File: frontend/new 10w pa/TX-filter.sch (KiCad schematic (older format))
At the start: 48 parts, among them K2 D3002, K3 D3002, K4 D3002, K5 D3002, K6 D3002, P8 CONN_01X08, U3 TPIC6B595, U4 TPIC6B595

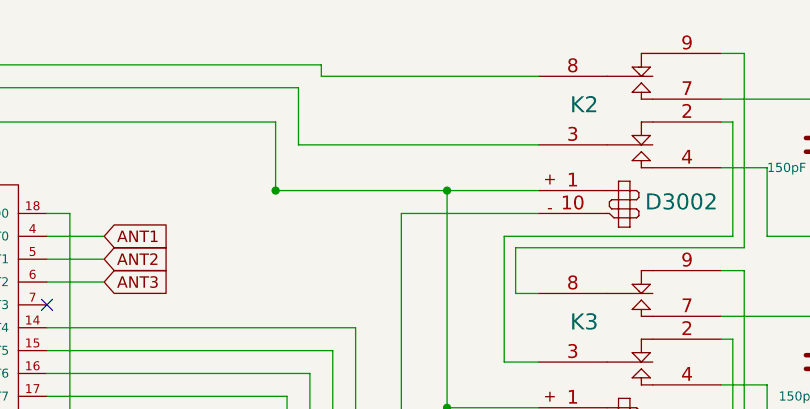
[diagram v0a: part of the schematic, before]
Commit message: More pcb changes
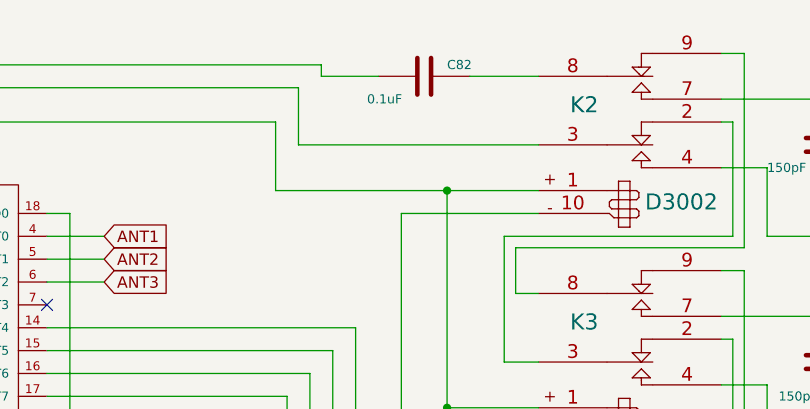
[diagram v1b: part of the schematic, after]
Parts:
- added C82: 0.1uF, HERMESLITE:C_0805, symbol C
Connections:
- net TXIN: now also C82.2; no longer K2.8 (C2)
- new net: C82.1, K2.8 (C2)
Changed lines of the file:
@@
 $EndComp
 $Comp
-L GND #PWR023
+L GND #PWR024
 U 1 1 5496A449
 P 6850 4150
-F 0 "#PWR023" H 6850 4150 30  0001 C CNN
+F 0 "#PWR024" H 6850 4150 30  0001 C CNN
 F 1 "GND" H 6850 4080 30  0001 C CNN
 F 2 "" H 6850 4150 60  0000 C CNN
@@
 $EndComp
 $Comp
-L GND #PWR024
+L GND #PWR025
 U 1 1 5496A44A
 P 5750 4150
-F 0 "#PWR024" H 5750 4150 30  0001 C CNN
+F 0 "#PWR025" H 5750 4150 30  0001 C CNN
 F 1 "GND" H 5750 4080 30  0001 C CNN
 F 2 "" H 5750 4150 60  0000 C CNN
@@
 $EndComp
 $Comp
-L GND #PWR025
+L GND #PWR026
 U 1 1 5496A44B
 P 7750 4150
-F 0 "#PWR025" H 7750 4150 30  0001 C CNN
+F 0 "#PWR026" H 7750 4150 30  0001 C CNN
 F 1 "GND" H 7750 4080 30  0001 C CNN
 F 2 "" H 7750 4150 60  0000 C CNN
@@
 	5400 4400 4400 4400
 $Comp
-L GND #PWR026
+L GND #PWR027
 U 1 1 5496A47D
 P 1900 5550
-F 0 "#PWR026" H 1900 5550 30  0001 C CNN
+F 0 "#PWR027" H 1900 5550 30  0001 C CNN
 F 1 "GND" H 1900 5480 30  0001 C CNN
 F 2 "" H 1900 5550 50  0000 C CNN
@@
 $EndComp
 $Comp
-L GND #PWR027
+L GND #PWR028
 U 1 1 54A155CF
 P 6800 5300
-F 0 "#PWR027" H 6800 5300 30  0001 C CNN
+F 0 "#PWR028" H 6800 5300 30  0001 C CNN
 F 1 "GND" H 6800 5230 30  0001 C CNN
 F 2 "" H 6800 5300 60  0000 C CNN
@@
 $EndComp
 $Comp
-L GND #PWR028
+L GND #PWR029
 U 1 1 54A1568D
 P 7400 5300
-F 0 "#PWR028" H 7400 5300 30  0001 C CNN
+F 0 "#PWR029" H 7400 5300 30  0001 C CNN
 F 1 "GND" H 7400 5230 30  0001 C CNN
 F 2 "" H 7400 5300 60  0000 C CNN
@@
 $EndComp
 $Comp
-L GND #PWR029
+L GND #PWR030
 U 1 1 54A171EB
 P 5950 6400
-F 0 "#PWR029" H 5950 6400 30  0001 C CNN
+F 0 "#PWR030" H 5950 6400 30  0001 C CNN
 F 1 "GND" H 5950 6330 30  0001 C CNN
 F 2 "" H 5950 6400 60  0000 C CNN
@@
 $EndComp
 $Comp
-L GND #PWR030
+L GND #PWR031
 U 1 1 54A171F1
 P 6550 6400
-F 0 "#PWR030" H 6550 6400 30  0001 C CNN
+F 0 "#PWR031" H 6550 6400 30  0001 C CNN
 F 1 "GND" H 6550 6330 30  0001 C CNN
 F 2 "" H 6550 6400 60  0000 C CNN
@@
 $EndComp
 $Comp
-L GND #PWR031
+L GND #PWR032
 U 1 1 54A1B96C
 P 6650 3200
-F 0 "#PWR031" H 6650 3200 30  0001 C CNN
+F 0 "#PWR032" H 6650 3200 30  0001 C CNN
 F 1 "GND" H 6650 3130 30  0001 C CNN
 F 2 "" H 6650 3200 60  0000 C CNN
@@
 $EndComp
 $Comp
-L GND #PWR032
+L GND #PWR033
 U 1 1 54A1B972
 P 5750 3200
-F 0 "#PWR032" H 5750 3200 30  0001 C CNN
+F 0 "#PWR033" H 5750 3200 30  0001 C CNN
 F 1 "GND" H 5750 3130 30  0001 C CNN
 F 2 "" H 5750 3200 60  0000 C CNN
@@
 $EndComp
 $Comp
-L GND #PWR033
+L GND #PWR034
 U 1 1 54A1B978
 P 7550 3200
-F 0 "#PWR033" H 7550 3200 30  0001 C CNN
+F 0 "#PWR034" H 7550 3200 30  0001 C CNN
 F 1 "GND" H 7550 3130 30  0001 C CNN
 F 2 "" H 7550 3200 60  0000 C CNN
@@
 $EndComp
 $Comp
-L GND #PWR034
+L GND #PWR035
 U 1 1 54A1CC1F
 P 6850 2250
-F 0 "#PWR034" H 6850 2250 30  0001 C CNN
+F 0 "#PWR035" H 6850 2250 30  0001 C CNN
 F 1 "GND" H 6850 2180 30  0001 C CNN
 F 2 "" H 6850 2250 60  0000 C CNN
@@
 $EndComp
 $Comp
-L GND #PWR035
+L GND #PWR036
 U 1 1 54A1CC25
 P 5950 2250
-F 0 "#PWR035" H 5950 2250 30  0001 C CNN
+F 0 "#PWR036" H 5950 2250 30  0001 C CNN
 F 1 "GND" H 5950 2180 30  0001 C CNN
 F 2 "" H 5950 2250 60  0000 C CNN
@@
 $EndComp
 $Comp
-L GND #PWR036
+L GND #PWR037
 U 1 1 54A1CC2B
 P 7750 2250
-F 0 "#PWR036" H 7750 2250 30  0001 C CNN
+F 0 "#PWR037" H 7750 2250 30  0001 C CNN
 F 1 "GND" H 7750 2180 30  0001 C CNN
 F 2 "" H 7750 2250 60  0000 C CNN
@@
 $EndComp
 $Comp
-L GND #PWR037
+L GND #PWR038
 U 1 1 54A1CDA5
 P 6650 1300
-F 0 "#PWR037" H 6650 1300 30  0001 C CNN
+F 0 "#PWR038" H 6650 1300 30  0001 C CNN
 F 1 "GND" H 6650 1230 30  0001 C CNN
 F 2 "" H 6650 1300 60  0000 C CNN
@@
 $EndComp
 $Comp
-L GND #PWR038
+L GND #PWR039
 U 1 1 54A1CDAB
 P 5750 1300
-F 0 "#PWR038" H 5750 1300 30  0001 C CNN
+F 0 "#PWR039" H 5750 1300 30  0001 C CNN
 F 1 "GND" H 5750 1230 30  0001 C CNN
 F 2 "" H 5750 1300 60  0000 C CNN
@@
 $EndComp
 $Comp
-L GND #PWR039
+L GND #PWR040
 U 1 1 54A1CDB1
 P 7550 1300
-F 0 "#PWR039" H 7550 1300 30  0001 C CNN
+F 0 "#PWR040" H 7550 1300 30  0001 C CNN
 F 1 "GND" H 7550 1230 30  0001 C CNN
 F 2 "" H 7550 1300 60  0000 C CNN
@@
 	1900 2450 1900 2500
 $Comp
-L GND #PWR040
+L GND #PWR041
 U 1 1 54A26C24
 P 1900 2500
-F 0 "#PWR040" H 1900 2500 30  0001 C CNN
+F 0 "#PWR041" H 1900 2500 30  0001 C CNN
 F 1 "GND" H 1900 2430 30  0001 C CNN
 F 2 "" H 1900 2500 60  0000 C CNN
@@
 	1900 4150 1900 4250
 $Comp
-L GND #PWR041
+L GND #PWR042
 U 1 1 54A272E7
 P 1900 4250
-F 0 "#PWR041" H 1900 4250 30  0001 C CNN
+F 0 "#PWR042" H 1900 4250 30  0001 C CNN
 F 1 "GND" H 1900 4180 30  0001 C CNN
 F 2 "" H 1900 4250 60  0000 C CNN
@@
 $EndComp
 $Comp
-L GND #PWR042
+L GND #PWR043
 U 1 1 54A63C22
 P 5950 4150
-F 0 "#PWR042" H 5950 4150 30  0001 C CNN
+F 0 "#PWR043" H 5950 4150 30  0001 C CNN
 F 1 "GND" H 5950 4080 30  0001 C CNN
 F 2 "" H 5950 4150 60  0000 C CNN
@@
 Connection ~ 7950 3750
 $Comp
-L GND #PWR043
+L GND #PWR044
 U 1 1 54A64006
 P 7950 4150
-F 0 "#PWR043" H 7950 4150 30  0001 C CNN
+F 0 "#PWR044" H 7950 4150 30  0001 C CNN
 F 1 "GND" H 7950 4080 30  0001 C CNN
 F 2 "" H 7950 4150 60  0000 C CNN
@@
 	3550 750  3550 800
 Wire Wire Line
-	3550 800  4500 800
-Wire Wire Line
 	3450 850  3450 1100
 Wire Wire Line
@@
 Wire Wire Line
 	3350 1300 4500 1300
-Connection ~ 3350 1300
 Wire Wire Line
 	4400 1550 4400 1750
@@
 $EndComp
 $Comp
-L GND #PWR044
+L GND #PWR045
 U 1 1 54ABE5DE
 P 5750 2250
-F 0 "#PWR044" H 5750 2250 30  0001 C CNN
+F 0 "#PWR045" H 5750 2250 30  0001 C CNN
 F 1 "GND" H 5750 2180 30  0001 C CNN
 F 2 "" H 5750 2250 60  0000 C CNN
@@
 $EndComp
 $Comp
-L GND #PWR045
+L GND #PWR046
 U 1 1 54ABE6E0
 P 8000 2250
-F 0 "#PWR045" H 8000 2250 30  0001 C CNN
+F 0 "#PWR046" H 8000 2250 30  0001 C CNN
 F 1 "GND" H 8000 2180 30  0001 C CNN
 F 2 "" H 8000 2250 60  0000 C CNN
@@
 Connection ~ 8000 1850
 Connection ~ 5750 1850
+$Comp
+L C C82
+U 1 1 54BBBF4C
+P 4000 800
+F 0 "C82" V 3950 900 40  0000 L CNN
+F 1 "0.1uF" V 4100 550 40  0000 L CNN
+F 2 "HERMESLITE:C_0805" H 4038 650 30  0001 C CNN
+F 3 "" H 4000 800 60  0000 C CNN
+	1    4000 800
+	0    1    1    0
+$EndComp
+Wire Wire Line
+	3550 800  3800 800
+Wire Wire Line
+	4200 800  4500 800
 $EndSCHEMATC

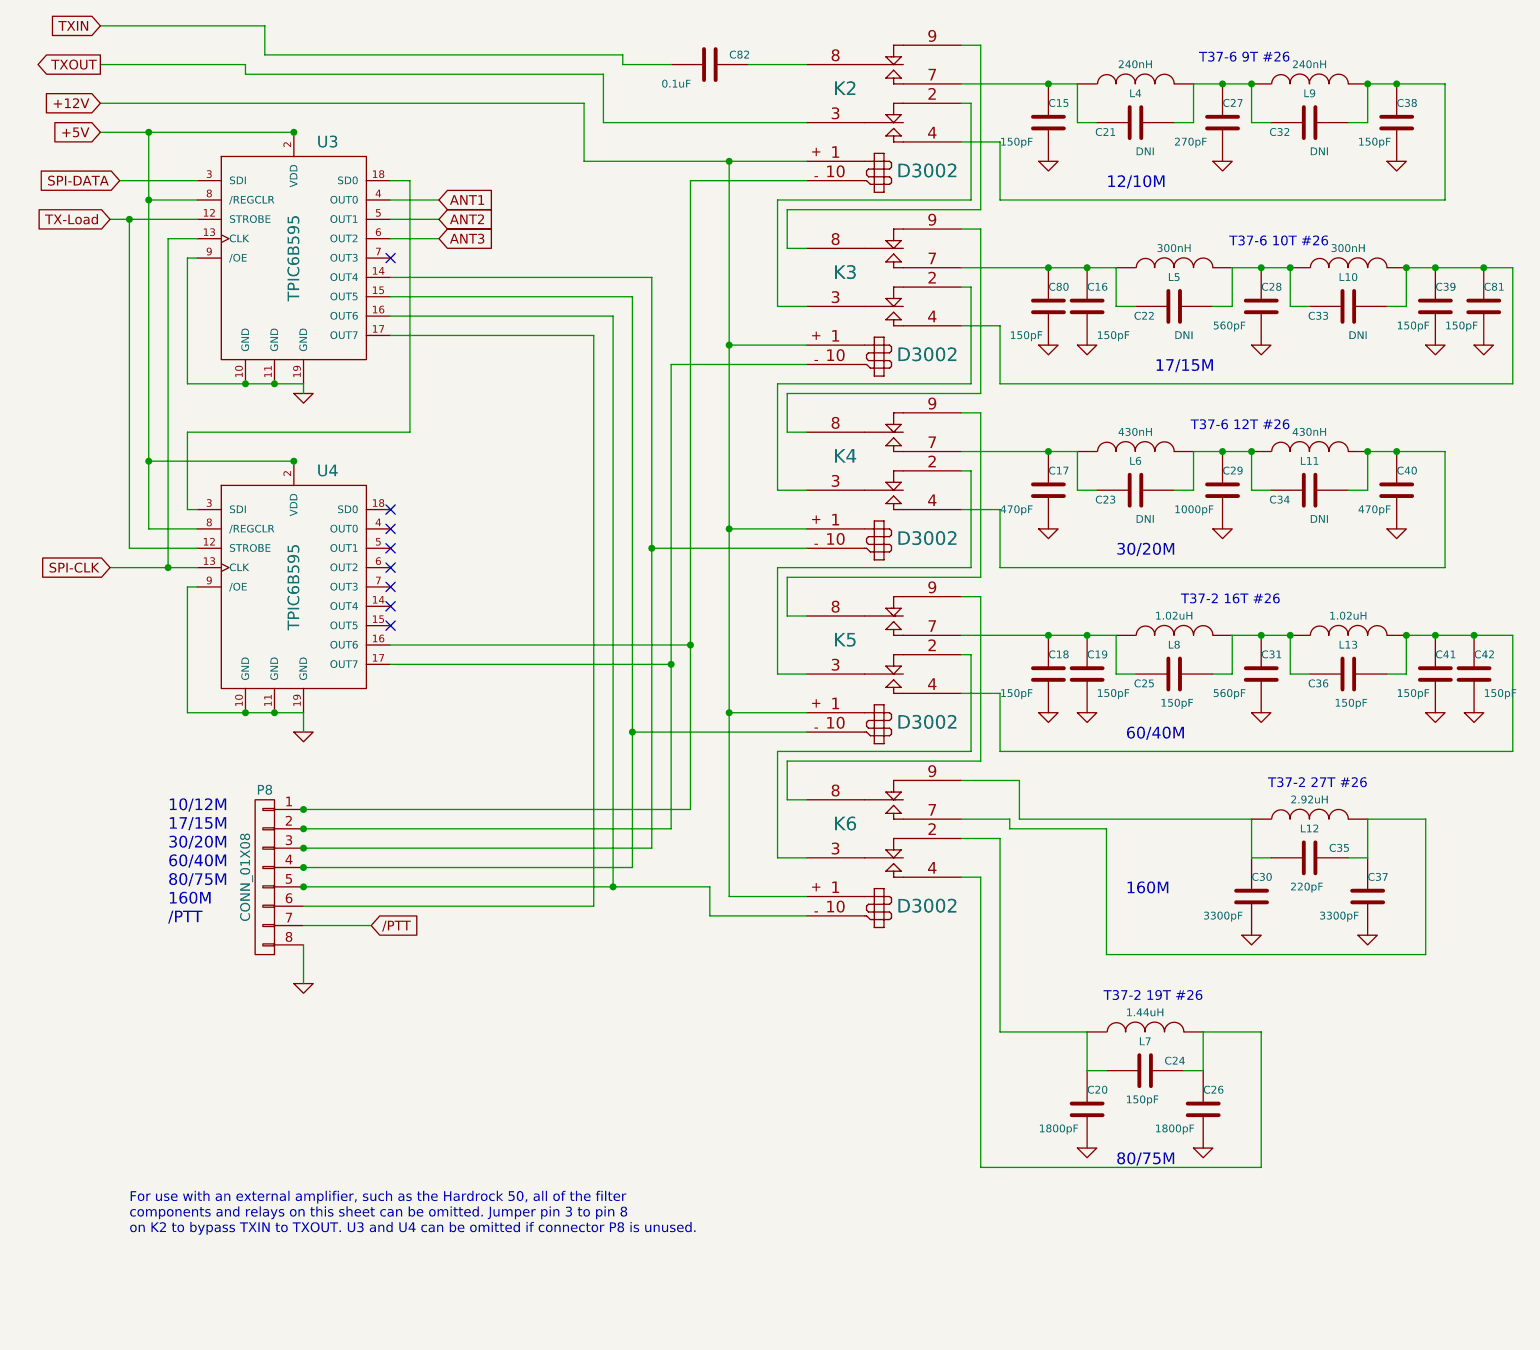
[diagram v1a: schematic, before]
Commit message: BCD Filter update
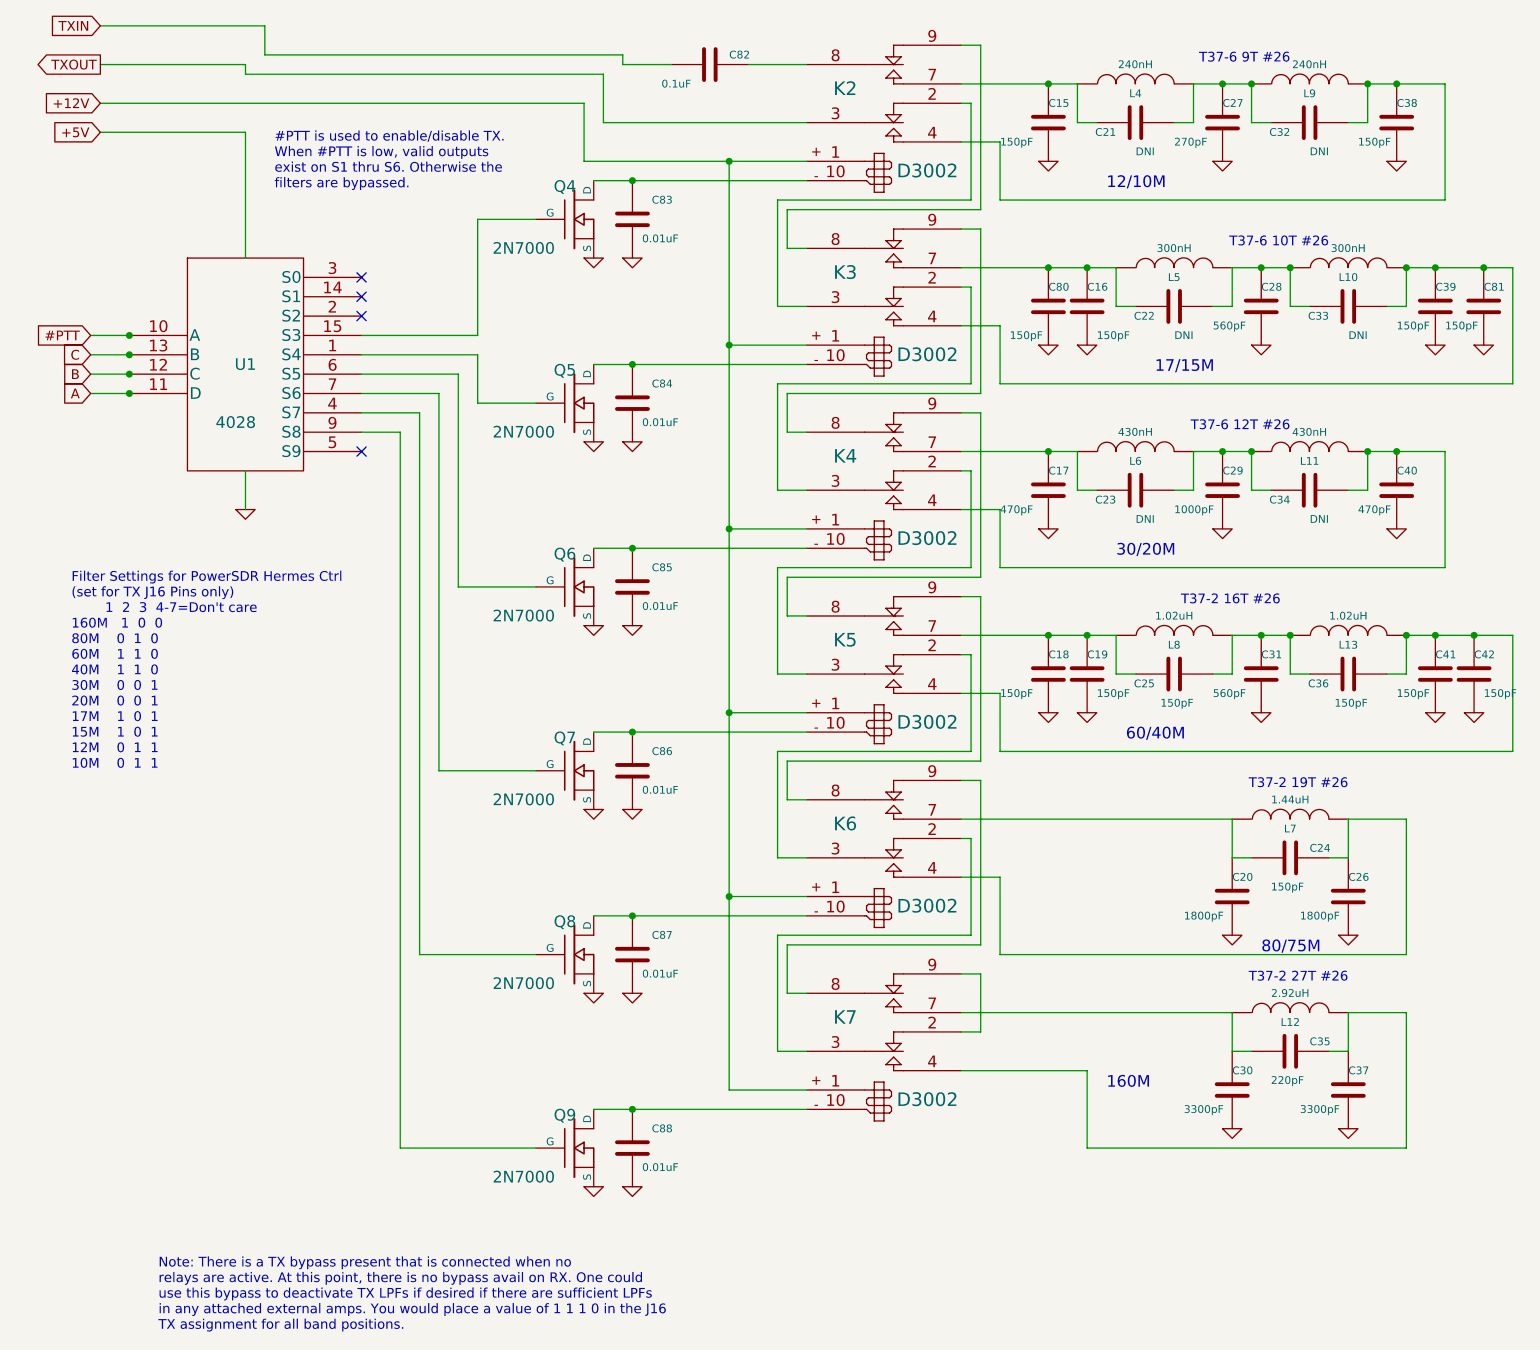
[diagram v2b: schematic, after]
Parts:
- removed P8: CONN_01X08, Pin_Headers:Pin_Header_Straight_1x08, symbol CONN_01X08
- removed U3, U4: TPIC6B595, Housings_SOIC:SOIC-20_7.5x12.8mm_Pitch1.27mm, symbol TPIC6B595
- added C83, C84, C85, C86, C87, C88: 0.01uF, HERMESLITE:C_0805, symbol C
- added K7: D3002, HERMESLITE:D3002, symbol D3002
- added Q4, Q5, Q6, Q7, Q8, Q9: 2N7000, SMD_Packages:SOT-23-GDS, symbol MOSFET_N
- added U1: 4028, SMD_Packages:TSSOP-16, symbol 4028
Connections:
- net +12V: now also K7.1 (+)
- net GND: now also C83.2, C84.2, C85.2, C86.2, C87.2, C88.2, Q4.2 (S), Q5.2 (S), Q6.2 (S), Q7.2 (S), Q8.2 (S), Q9.2 (S), U1.8 (VSS)
- net at C35.1, C37.1, L12.2: now also K7.4 (T1); no longer K6.7 (T2)
- net at C30.1, C35.2, L12.1: now also K7.7 (T2); no longer K6.9 (R2)
- net at K2.10 (-): now also C83.1, Q4.3 (D)
- net at K3.10 (-): now also C84.1, Q5.3 (D)
- net at K4.10 (-): now also C85.1, Q6.3 (D)
- net at K5.10 (-): now also C86.1, Q7.3 (D)
- net at K6.10 (-): now also C87.1, Q8.3 (D)
- net at C20.1, C24.2, L7.1: now also K6.7 (T2); no longer K6.2 (R1)
- new net: K6.2 (R1), K7.3 (C1)
- new net: K6.9 (R2), K7.8 (C2)
- new net: C88.1, K7.10 (-), Q9.3 (D)
- new net: K7.2 (R1), K7.9 (R2)
- new net: Q9.1 (G), U1.9 (S8)
- new net: Q8.1 (G), U1.4 (S7)
- new net: Q7.1 (G), U1.7 (S6)
- new net: Q6.1 (G), U1.6 (S5)
- new net: Q5.1 (G), U1.1 (S4)
- new net: Q4.1 (G), U1.15 (S3)
- new net #PTT: U1.10 (A)
- new net A: U1.11 (D)
- new net B: U1.12 (C)
- new net C: U1.13 (B)
- new net VDD: U1.16 (VDD)
- no-connect marks 8 -> 4
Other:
- note added: "#PTT is used to enable/disable TX. \nWhen #PTT is low, valid outputs\nexist on S1 thru S6. Otherwise the \nfilters are bypassed."
- note added: "Filter Settings for PowerSDR Hermes Ctrl\n(set for TX J16 Pins only)\n 1 2 3 4-7=Don't care\n160M 1 0 0\n80M 0 1 0\n60M 1 1 0\n40M 1 1 0\n30M 0 0 1\n20M 0 0 1\n17M 1 0 1\n15M 1 0 1\n12M 0 1 1\n10M 0 1 1"
- note added: "Note: There is a TX bypass present that is connected when no \nrelays are active. At this point, there is no bypass avail on RX. One could \nuse this bypass to deactivate TX LPFs if desired if there are sufficient LPFs \nin any attached external amps. You would place a value of 1 1 1 0 in the J16 \nTX assignment for all band positions."
- note removed: "10/12M\n17/15M\n30/20M\n60/40M\n80/75M\n160M\n/PTT"
- note removed: "For use with an external amplifier, such as the Hardrock 50, all of the filter\ncomponents and relays on this sheet can be omitted. Jumper pin 3 to pin 8\non K2 to bypass TXIN to TXOUT. U3 and U4 can be omitted if connector P8 is unused."
- moved on the sheet: C20, C24, C26, C30, C35, C37, L12, L7
